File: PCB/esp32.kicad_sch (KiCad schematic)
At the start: 29 parts, among them J1 UART, SW1 Boot, SW2 Reset, U4 ESP32-S3-WROOM-1, U8 GT-USB-7010ASV, U9 SGM2212-3.3XKC3G

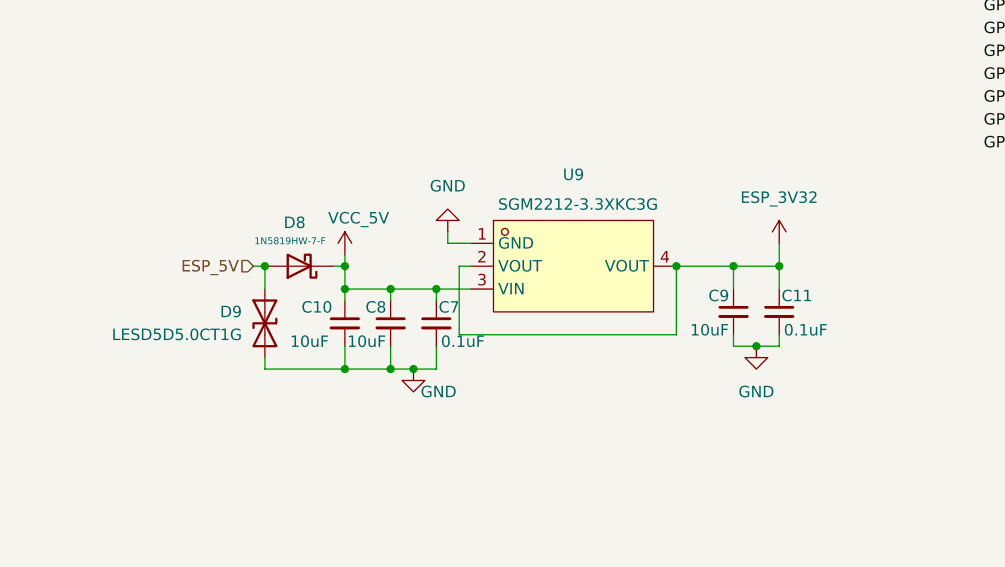
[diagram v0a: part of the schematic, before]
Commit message: Initial commit of project source code
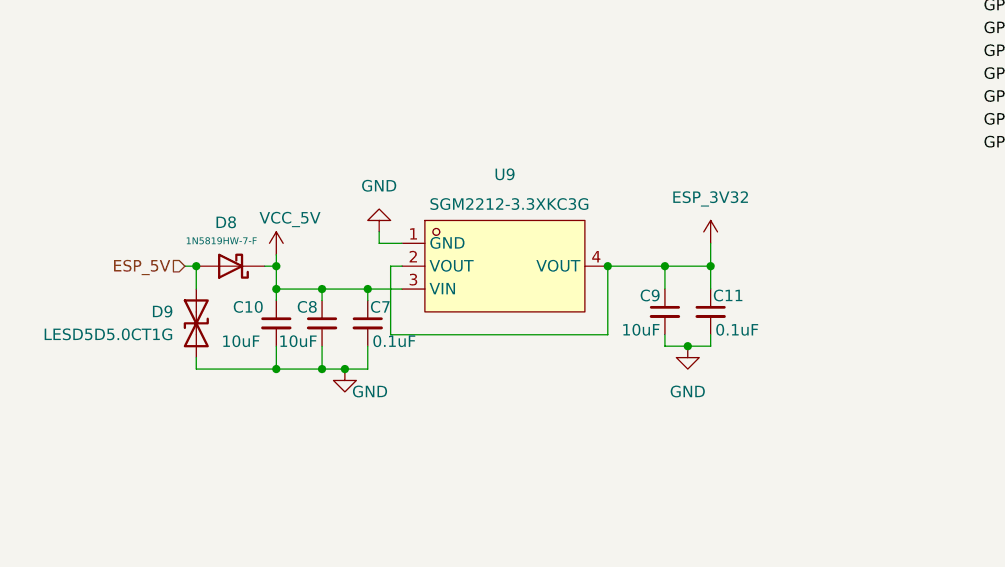
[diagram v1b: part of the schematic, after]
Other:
- moved on the sheet: C10, C11, C7, C8, C9, D8, D9, U9
